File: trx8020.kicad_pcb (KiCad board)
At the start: 2 copper layers, 78 parts, among them IC1 NE5534, IC2 78L10, IC3 78L06, IC4 SA612, IC5 SA612, IC6 78L06, IC7 78L05, IC8 AD9850, IC9 78Lxx, J1 Pin_1x6, M1 Mic, Q1 6 MHz, Q2 6MHz, Q3 6MHz, Q4 6MHz, Q5 6MHz, T1 BC-547

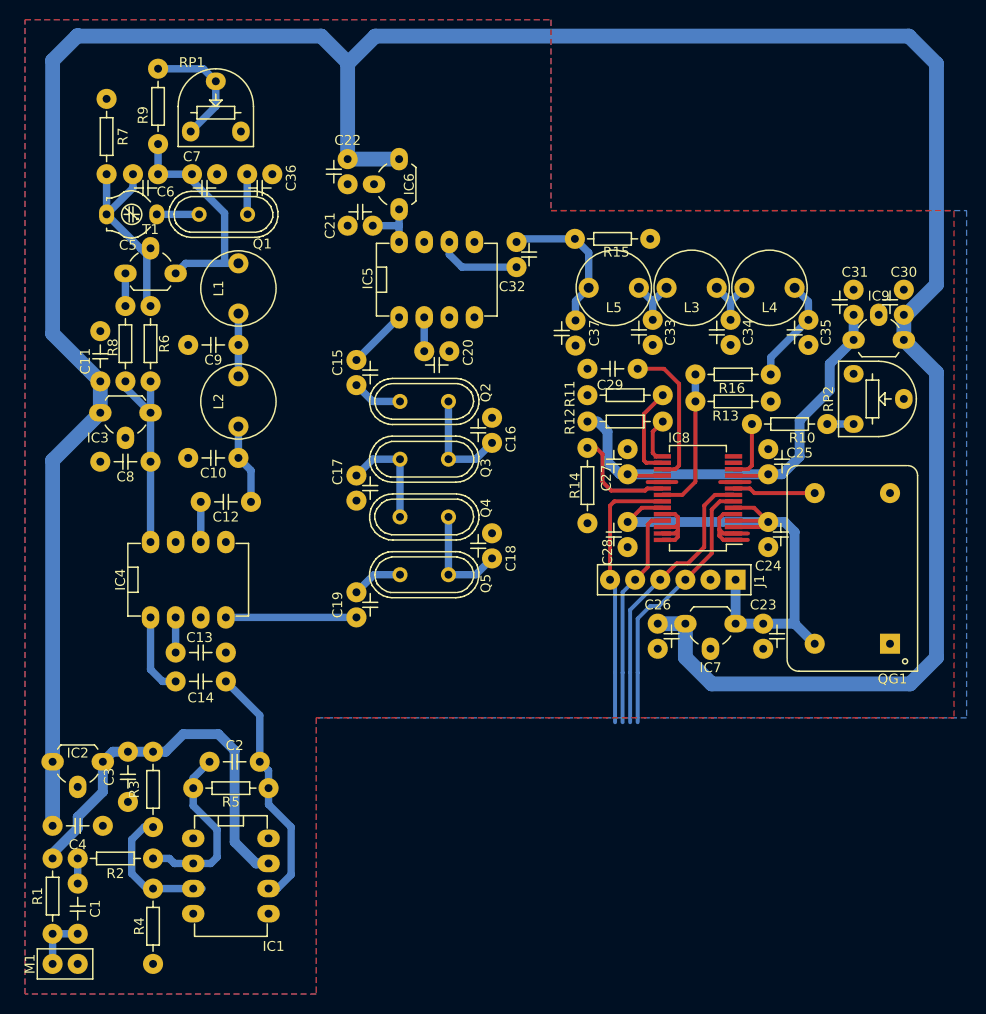
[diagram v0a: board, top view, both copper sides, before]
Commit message: minor fix
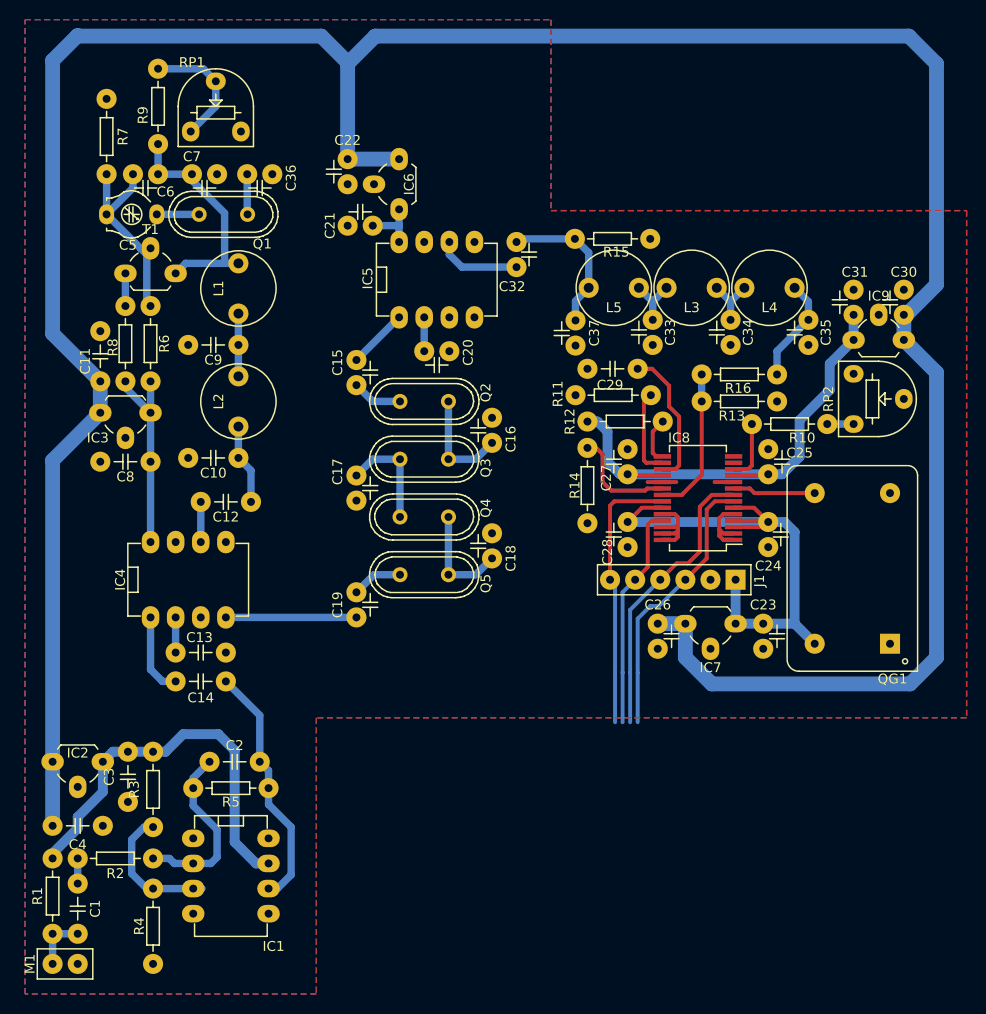
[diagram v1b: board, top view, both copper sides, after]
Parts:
- moved R11 1.21 mm to (77.3, 132.5)
- moved R13 0.64 mm to (90.0, 133.1)
- moved R16 0.64 mm to (90.0, 130.4)
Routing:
- net GND: track 24.2 -> 20.2 mm
- net Net-(C29-Pad1): track 14.9 -> 14.2 mm
